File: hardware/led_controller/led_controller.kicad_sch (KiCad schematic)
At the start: 32 parts, among them J1 Header, J2 Header, J3 Header, J4 Header, J5 POWER, J6 Conn_01x02, U1 74AHCT125, U3 Waveshare ESP32-S3/C6 Zero

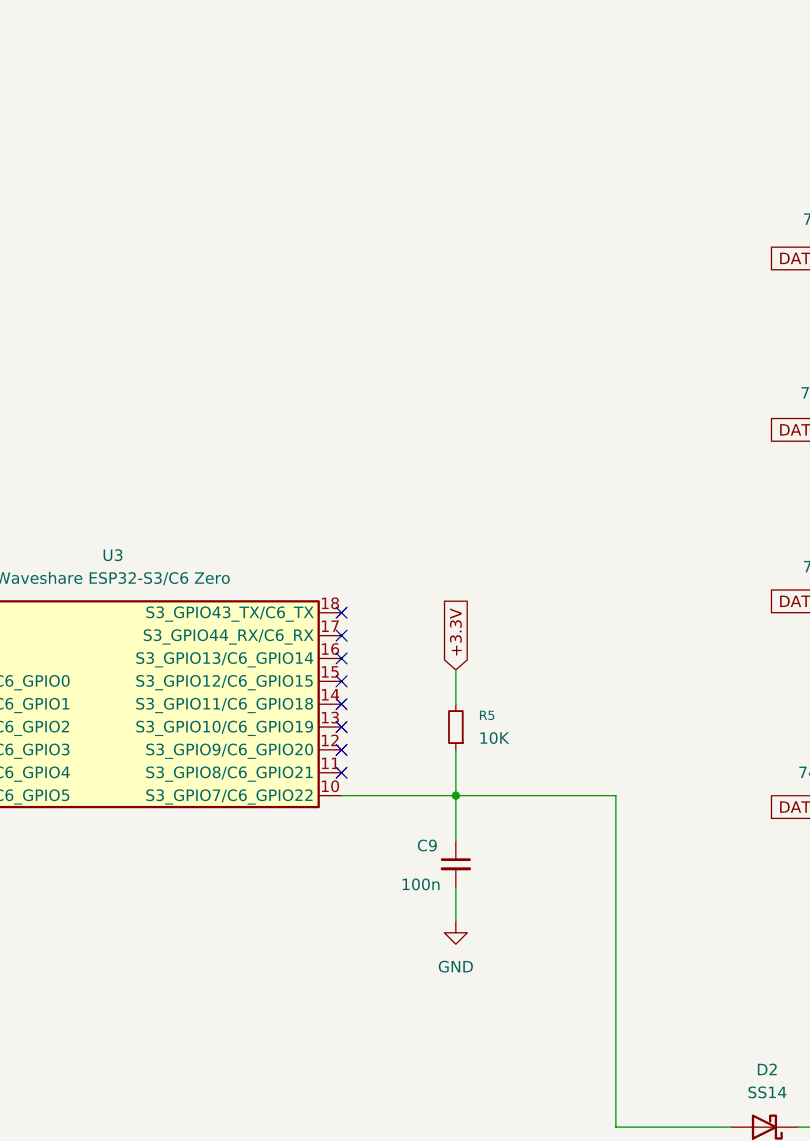
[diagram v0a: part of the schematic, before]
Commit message: PCB updates + fudicials fix
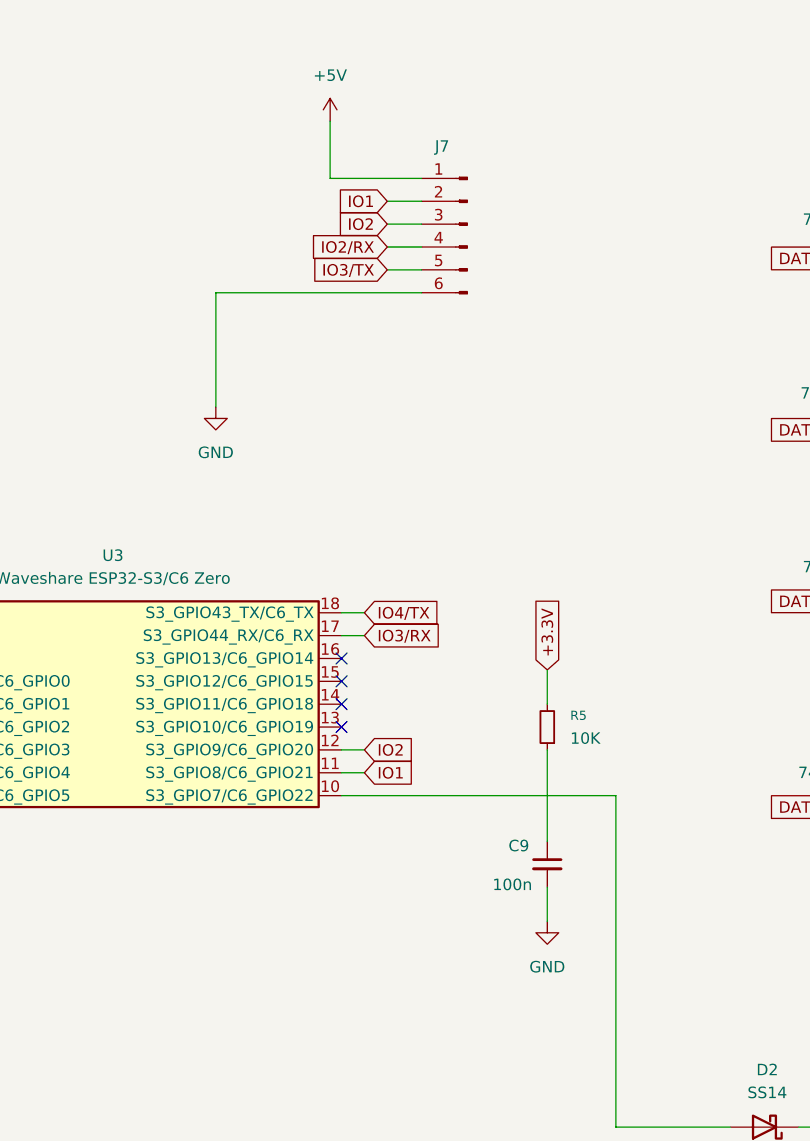
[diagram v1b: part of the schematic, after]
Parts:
- added J7: Conn_01x06_Pin, Connector_PinHeader_2.54mm:PinHeader_1x06_P2.54mm_Vertical, symbol Connector:Conn_01x06_Pin
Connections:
- net +5V: now also J7.1 (Pin_1)
- net GND: now also J7.6 (Pin_6)
- net at D2.2 (A), U3.10 (S3_GPIO7/C6_GPIO22): no longer C9.1, R5.1
- net IO1: now reaches U3.11 (S3_GPIO8/C6_GPIO21)
- net IO1: now also J7.2 (Pin_2)
- net IO2: now reaches U3.12 (S3_GPIO9/C6_GPIO20)
- net IO2: now also J7.3 (Pin_3)
- net IO3/RX: now reaches U3.17 (S3_GPIO44_RX/C6_RX)
- net IO4/TX: now reaches U3.18 (S3_GPIO43_TX/C6_TX)
- new net: C9.1, R5.1
- new net IO2/RX: J7.4 (Pin_4)
- new net IO3/TX: J7.5 (Pin_5)
- no-connect marks 14 -> 10
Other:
- moved on the sheet: C9, R5

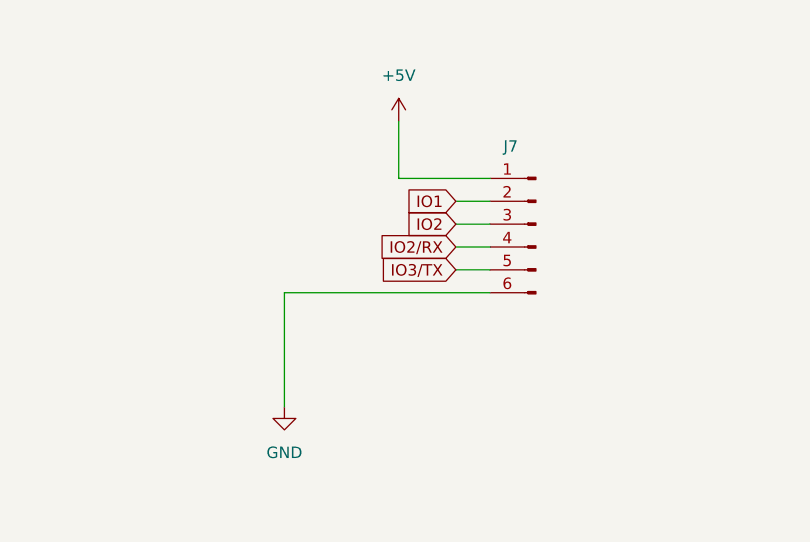
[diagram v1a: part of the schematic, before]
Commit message: Boards ordered v1.0
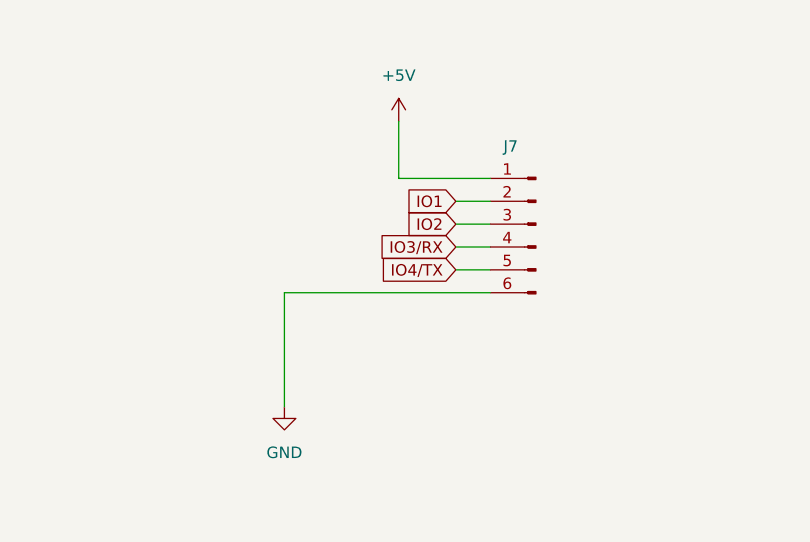
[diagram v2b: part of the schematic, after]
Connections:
- net IO2/RX is gone; now on net IO3/RX: J7.4 (Pin_4)
- net IO3/TX is gone; now on net IO4/TX: J7.5 (Pin_5)
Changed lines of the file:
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@@
 		)
 	)
-	(global_label "IO2{slash}RX"
+	(global_label "IO3{slash}RX"
 		(shape input)
 		(at 140.97 43.18 180)
@@
 		)
 	)
-	(global_label "IO3{slash}TX"
+	(global_label "IO4{slash}TX"
 		(shape input)
 		(at 140.97 45.72 180)
